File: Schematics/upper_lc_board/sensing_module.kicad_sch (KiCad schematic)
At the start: 13 parts, among them J5 HALL-1, U7 ADC_ADS131M04IPWR

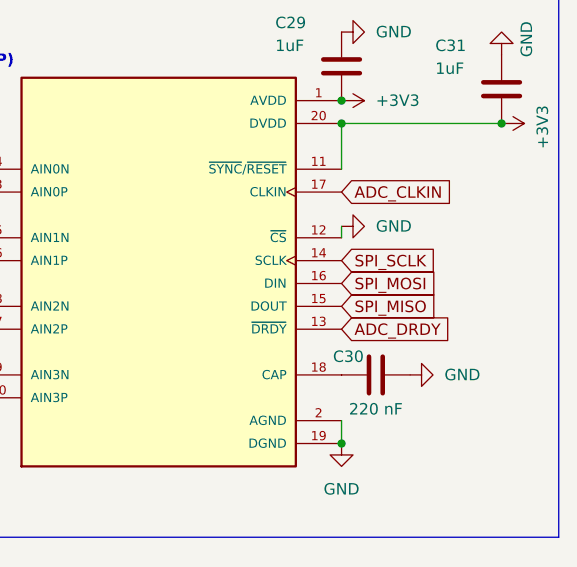
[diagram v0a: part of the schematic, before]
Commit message: add ed pinouts
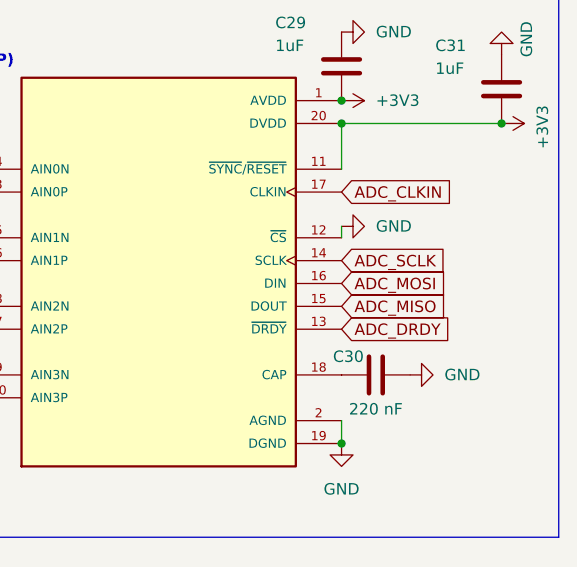
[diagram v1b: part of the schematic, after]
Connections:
- net SPI_MISO renamed ADC_MISO
- net SPI_MOSI renamed ADC_MOSI
- net SPI_SCLK renamed ADC_SCLK
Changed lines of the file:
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@@
 		)
 	)
-	(global_label "SPI_MOSI"
+	(global_label "ADC_MOSI"
 		(shape input)
 		(at 213.36 77.47 0)
@@
 		)
 		(property "Intersheetrefs" "${INTERSHEET_REFS}"
-			(at 224.9933 77.47 0)
+			(at 225.5376 77.47 0)
 			(effects
 				(font
@@
 		)
 	)
-	(global_label "SPI_MISO"
+	(global_label "ADC_MISO"
 		(shape input)
 		(at 213.36 80.01 0)
@@
 		)
 		(property "Intersheetrefs" "${INTERSHEET_REFS}"
-			(at 224.9933 80.01 0)
+			(at 225.5376 80.01 0)
 			(effects
 				(font
@@
 		)
 	)
-	(global_label "SPI_SCLK"
+	(global_label "ADC_SCLK"
 		(shape input)
 		(at 213.36 74.93 0)
@@
 		)
 		(property "Intersheetrefs" "${INTERSHEET_REFS}"
-			(at 225.1747 74.93 0)
+			(at 225.719 74.93 0)
 			(effects
 				(font
